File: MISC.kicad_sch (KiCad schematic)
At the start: 18 parts

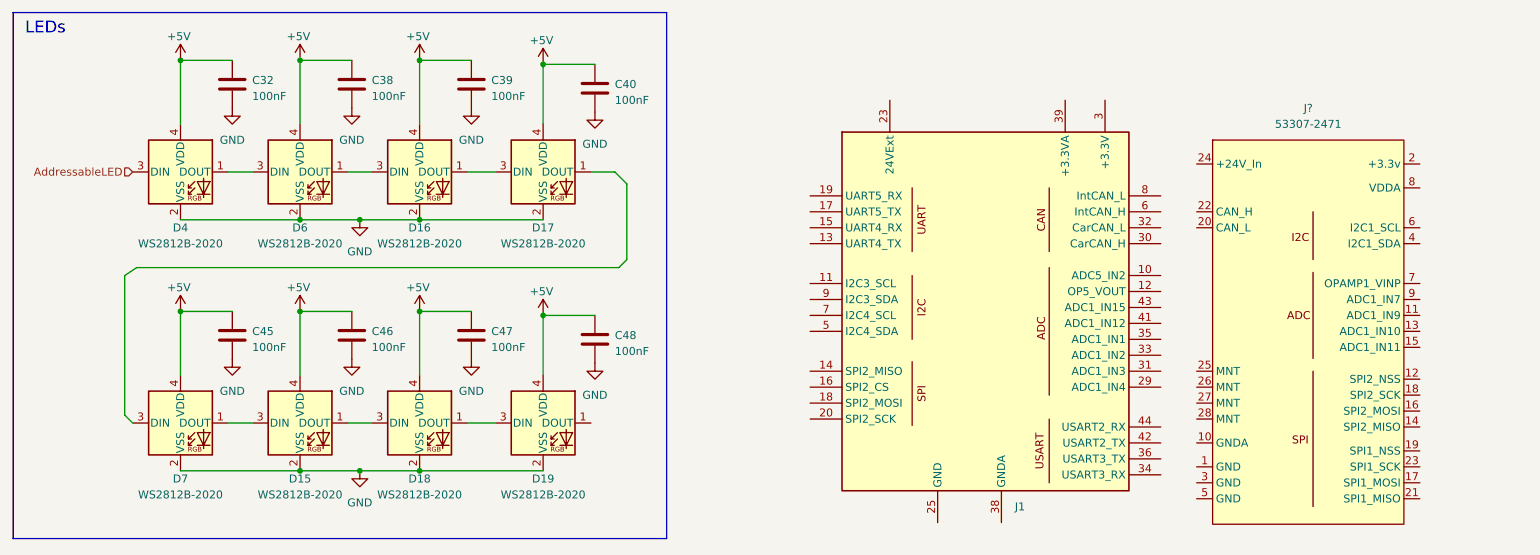
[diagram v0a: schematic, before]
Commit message: review council stuff
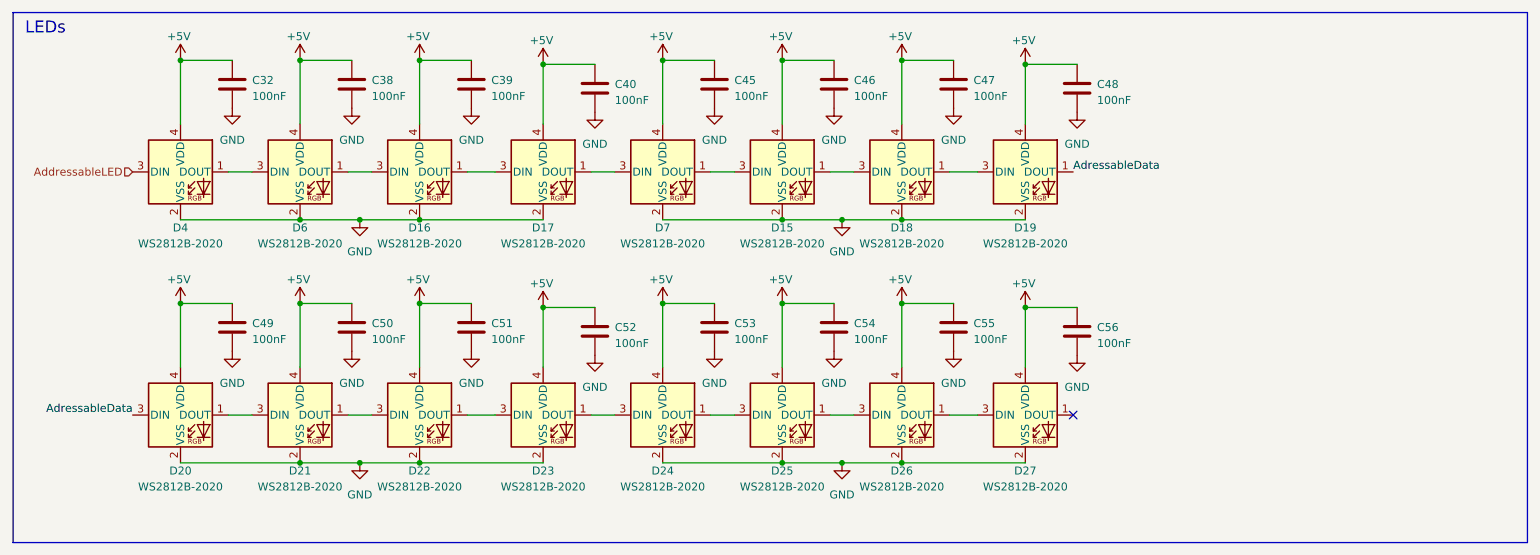
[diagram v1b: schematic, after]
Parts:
- removed J1: ~, symbol UTSVT-Connectors:LSOM_DaughterConn
- removed J?: 53307-2471, UTSVT_Connectors:PeripheralSOM, symbol UTSVT-Connectors:PeripheralSOMConnector
- added C49, C50, C51, C52, C53, C54, C55, C56: 100nF, Capacitor_SMD:C_0603_1608Metric_Pad1.08x0.95mm_HandSolder, symbol Device:C
- added D20, D21, D22, D23, D24, D25, D26, D27: WS2812B-2020, LED_SMD:LED_WS2812B-2020_PLCC4_2.0x2.0mm, symbol LED:WS2812B-2020
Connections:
- net +5V: now also C49.1, C50.1, C51.1, C52.1, C53.1, C54.1, C55.1, C56.1, D20.4 (VDD), D21.4 (VDD), D22.4 (VDD), D23.4 (VDD), D24.4 (VDD), D25.4 (VDD), D26.4 (VDD), D27.4 (VDD)
- net GND: now also C49.2, C50.2, C51.2, C52.2, C53.2, C54.2, C55.2, C56.2, D20.2 (VSS), D21.2 (VSS), D22.2 (VSS), D23.2 (VSS), D24.2 (VSS), D25.2 (VSS), D26.2 (VSS), D27.2 (VSS)
- net AdressableData: now reaches D19.1 (DOUT)
- net AdressableData: now also D20.3 (DIN)
- new net: D22.1 (DOUT), D23.3 (DIN)
- new net: D21.1 (DOUT), D22.3 (DIN)
- new net: D25.1 (DOUT), D26.3 (DIN)
- new net: D24.1 (DOUT), D25.3 (DIN)
- new net: D20.1 (DOUT), D21.3 (DIN)
- new net: D23.1 (DOUT), D24.3 (DIN)
- new net: D26.1 (DOUT), D27.3 (DIN)
- no-connect marks 0 -> 1
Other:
- moved on the sheet: C45, C46, C47, C48, D15, D18, D19, D7
